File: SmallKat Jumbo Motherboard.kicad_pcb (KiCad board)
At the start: 4 copper layers, 80 x 80 mm, 49 parts, among them IC1 TPS562201DDCR, IC2 TPS562201DDCR, J1 Conn_01x06_Male, J10 Conn_01x06_Male, J11 Conn_01x06_Male, J12 Conn_01x05_Male, J13 Conn_01x02_Male, J14 Conn_01x04_Male, J15 Conn_01x04_Male, J16 Conn_01x06_Male, J2 Conn_01x06_Male, J3 Conn_01x06_Male, J4 Conn_01x06_Male, J5 Conn_01x06_Male, J6 Conn_01x06_Male, J7 Conn_01x06_Male, J8 Conn_01x06_Male, J9 Conn_01x06_Male, U1 STM32H753IITx, Y1 32.768khz, Y2 32MHZ

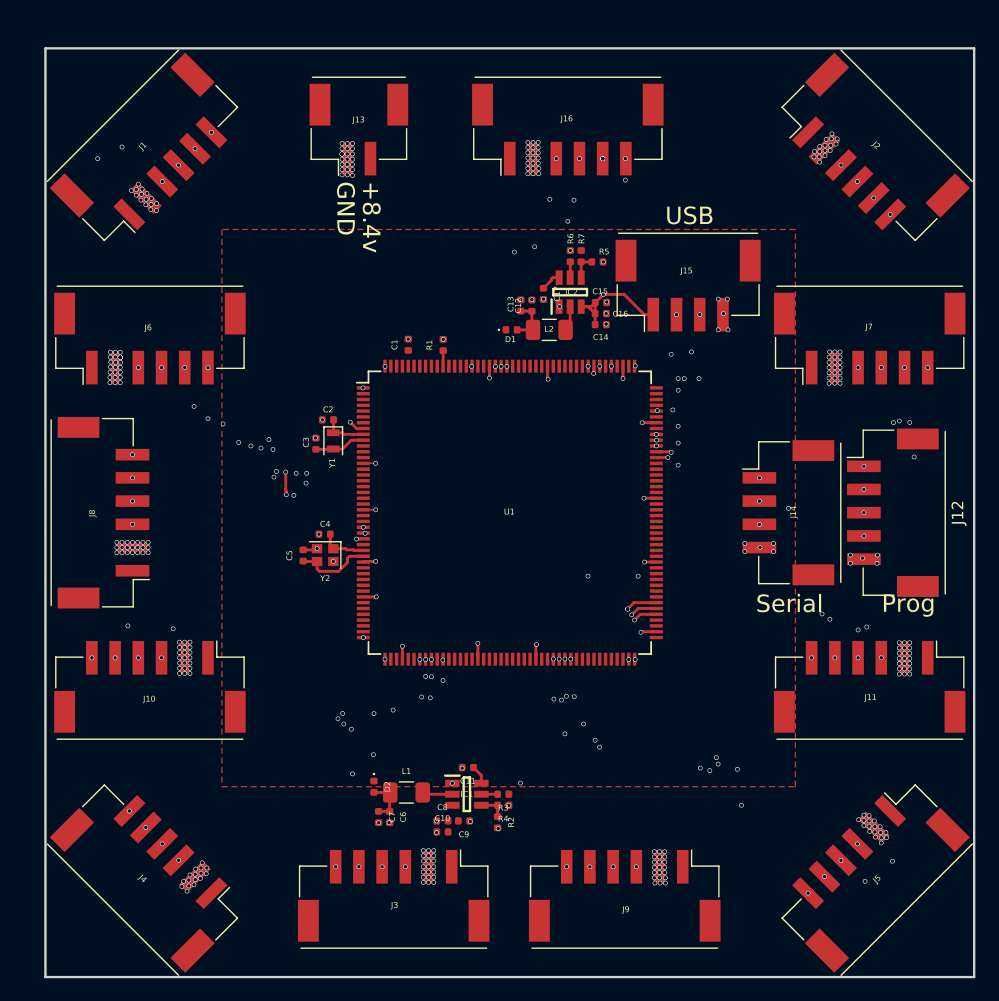
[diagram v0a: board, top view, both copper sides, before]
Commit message: Rev 2
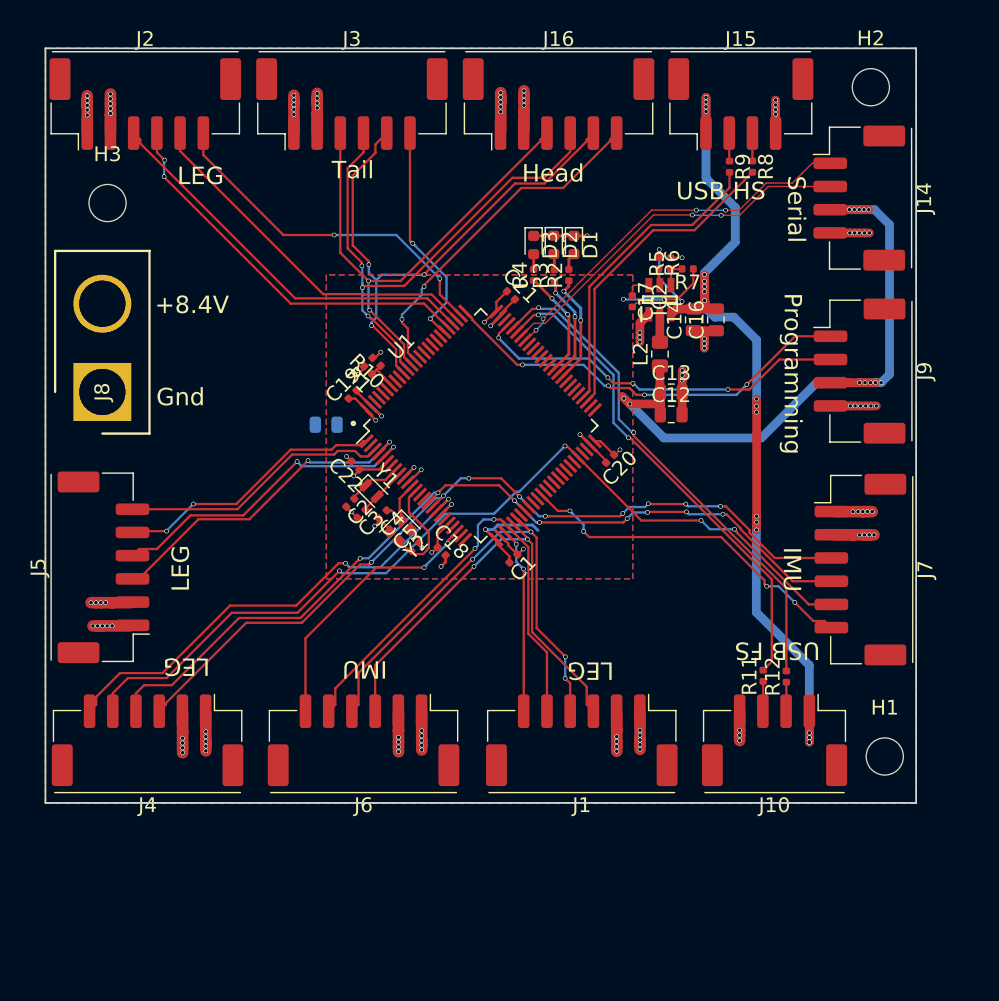
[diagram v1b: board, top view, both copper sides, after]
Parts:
- removed C10, C11: 0.1UF, Capacitor_SMD:C_0402_1005Metric
- removed C15, C8, C9: 10UF, Capacitor_SMD:C_0402_1005Metric
- removed C6, C7: 22UF, Capacitor_SMD:C_0402_1005Metric
- removed IC1: TPS562201DDCR, TPS562201DDCR:SOT95P280X110-6N
- removed J11: Conn_01x06_Male, Connector_Molex:Molex_CLIK-Mate_502443-0670_1x06-1MP_P2.00mm_Vertical
- removed J12: Conn_01x05_Male, Connector_Molex:Molex_CLIK-Mate_502443-0570_1x05-1MP_P2.00mm_Vertical
- removed J13: Conn_01x02_Male, Connector_Molex:Molex_CLIK-Mate_502443-0270_1x02-1MP_P2.00mm_Vertical
- removed L1: 4.7UH, Inductor_SMD:L_1206_3216Metric
- added C18: 0.1uF, Capacitor_SMD:C_0402_1005Metric, F.Cu at (34.1, 43.3)
- added C19: 0.1uF, Capacitor_SMD:C_0402_1005Metric, F.Cu at (26.5, 29.8)
- added C20: 0.1uF, Capacitor_SMD:C_0402_1005Metric, F.Cu at (48.6, 35.4)
- added C21: 0.1uF, Capacitor_SMD:C_0402_1005Metric, F.Cu at (40.1, 21.3)
- added C22: 0.1uF, Capacitor_SMD:C_0402_1005Metric, F.Cu at (26.7, 35.9)
- added D3: LED, LED_SMD:LED_0603_1608Metric, F.Cu at (42.1, 16.9)
- added FB1: Ferrite_Bead, Inductor_SMD:L_0805_2012Metric, B.Cu at (24.2, 32.4)
- added H1: MountingHole, MountingHole:MountingHole_3.2mm_M3, F.Cu at (72.3, 61.0)
- added H2: MountingHole, MountingHole:MountingHole_3.2mm_M3, F.Cu at (71.1, 3.35)
- added H3: MountingHole, MountingHole:MountingHole_3.2mm_M3, F.Cu at (5.35, 13.3)
- added R10: 10k, Resistor_SMD:R_0402_1005Metric, F.Cu at (28.5, 27.0)
- added R11: 33R, Resistor_SMD:R_0402_1005Metric, F.Cu at (61.8, 54.0)
- added R12: 33R, Resistor_SMD:R_0402_1005Metric, F.Cu at (63.8, 54.1)
- added R8: 33R, Resistor_SMD:R_0402_1005Metric, F.Cu at (60.9, 10.2)
- added R9: 33R, Resistor_SMD:R_0402_1005Metric, F.Cu at (58.9, 10.2)
- C1: value 1UF -> 0.1uF
- C12, C13, C14, C16: footprint Capacitor_SMD:C_0402_1005Metric -> Capacitor_SMD:C_0805_2012Metric
- D1, D2: value 641-1675-1-ND -> LED; footprint Diode_SMD:D_0402_1005Metric -> LED_SMD:LED_0603_1608Metric
- J10, J9: value Conn_01x06_Male -> Conn_01x04_Male; footprint Connector_Molex:Molex_CLIK-Mate_502443-0670_1x06-1MP_P2.00mm_Vertical -> Connector_Molex:Molex_CLIK-Mate_502443-0470_1x04-1MP_P2.00mm_Vertical
- J8: value Conn_01x06_Male -> PRT-10474; footprint Connector_Molex:Molex_CLIK-Mate_502443-0670_1x06-1MP_P2.00mm_Vertical -> PRT-10474:SHDR2W320P716_1X2_1574X813X1588P
- L2: footprint Inductor_SMD:L_1206_3216Metric -> Inductor_SMD:L_0805_2012Metric_Pad1.15x1.40mm_HandSolder
- R1, R5: value 10K -> 10k
- R2, R3: value 10K -> 330R
- R4: value 33.2K -> 330R
- R7: value 33.2K -> 33.2k
- U1: value STM32H753IITx -> STM32H743VITx; footprint Package_QFP:LQFP-176_24x24mm_P0.5mm -> Package_QFP:LQFP-100_14x14mm_P0.5mm
- moved J5 71.0 mm to (5.00, 44.7), turned to 90 degrees
- moved J3 68.3 mm to (26.4, 4.80), turned to 0 degrees
- moved J1 62.8 mm to (46.2, 59.6), turned to 180 degrees
- moved J2 62.5 mm to (8.60, 4.80), turned to 0 degrees
- moved J10 54.0 mm to (62.8, 59.6)
- moved J9 49.5 mm to (70.1, 27.8), turned to 270 degrees
- moved D2 49.2 mm to (43.8, 16.9)
- moved R2 47.5 mm to (45.1, 19.5), turned to 90 degrees
- moved R4 45.8 mm to (42.1, 19.5), turned to 90 degrees
- moved R3 44.9 mm to (43.8, 19.6), turned to 90 degrees
- moved J6 39.2 mm to (27.4, 59.6), turned to 180 degrees
- moved J14 27.8 mm to (70.1, 12.9)
- moved C1 20.5 mm to (40.3, 44.0), turned to 225 degrees
- moved J7 19.9 mm to (70.2, 44.9), turned to 270 degrees
- moved J15 16.3 mm to (59.9, 4.80)
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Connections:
- C1 pad 2: GND -> MCU_GND
- C12 pad 1: Net-(C12-Pad1) -> +3V3
- C13 pad 1: Net-(C12-Pad1) -> +3V3
- C17 pad 2: GND -> Net-(C17-Pad2)
- C2 pad 2: GND -> MCU_GND
- C3 pad 2: GND -> MCU_GND
- C4 pad 2: GND -> MCU_GND
- C5 pad 2: GND -> MCU_GND
- D1 pad 1: +3V3 -> GND
- D1 pad 2: Net-(C12-Pad1) -> Net-(D1-Pad2)
- D2 pad 1: +3V3 -> GND
- D2 pad 2: Net-(C6-Pad1) -> Net-(D2-Pad2)
- IC2 pad 2: Net-(IC2-Pad2) -> Net-(C17-Pad2)
- J1 pad 3: SCK1 -> MISO1
- J1 pad 4: MISO1 -> MOSI1
- J1 pad 5: MOSI1 -> SCK1
- J1 pad 6: CS1_1 -> CS1
- J10 pad 1: +BATT -> +5V
- J10 pad 2: GND -> Net-(J10-Pad2)
- J10 pad 3: SCK5 -> Net-(J10-Pad3)
- J10 pad 4: MISO5 -> GND
- J15 pad 2: USBDM -> Net-(J15-Pad2)
- J15 pad 3: USBDP -> Net-(J15-Pad3)
- J16 pad 6: CS6 -> CS6_HEAD
- J2 pad 3: SCK1 -> MISO3
- J2 pad 4: MISO1 -> MOSI3
- J2 pad 5: MOSI1 -> SCK3
- J2 pad 6: CS1_2 -> CS3
- J3 pad 3: SCK2 -> SCK6
- J3 pad 4: MISO2 -> MISO6
- J3 pad 5: MOSI2 -> MOSI6
- J3 pad 6: CS2 -> CS6_TAIL
- J4 pad 3: SCK1 -> MISO2
- J4 pad 4: MISO1 -> MOSI2
- J4 pad 5: MOSI1 -> SCK2
- J4 pad 6: CS1_3 -> CS2
- J5 pad 3: SCK1 -> MISO4
- J5 pad 4: MISO1 -> MOSI4
- J5 pad 5: MOSI1 -> SCK4
- J5 pad 6: CS1_4 -> CS4
- J6 pad 3: SCK5 -> MISO1
- J6 pad 4: MISO5 -> MOSI1
- J6 pad 5: MOSI5 -> SCK1
- J6 pad 6: CS5_1 -> IMU1_CS
- J7 pad 3: SCK5 -> MISO2
- J7 pad 4: MISO5 -> MOSI2
- J7 pad 5: MOSI5 -> SCK2
- J7 pad 6: CS5_2 -> IMU2_CS
- J8 pad 1: +BATT -> GND
- J8 pad 2: GND -> +BATT
- J9 pad 1: +BATT -> SWCLK
- J9 pad 2: GND -> SWDIO
- J9 pad 3: SCK4 -> +3V3
- J9 pad 4: MISO4 -> GND
- L2 pad 1: Net-(C12-Pad1) -> +3V3
- L2 pad 2: Net-(IC2-Pad2) -> Net-(C17-Pad2)
- R2 pad 1: Net-(IC1-Pad4) -> LED1
- R2 pad 2: GND -> Net-(D1-Pad2)
- R3 pad 1: +BATT -> LED2
- R3 pad 2: Net-(IC1-Pad5) -> Net-(D2-Pad2)
- R4 pad 1: +3V3 -> LED3
- R4 pad 2: Net-(IC1-Pad4) -> Net-(D3-Pad2)
- U1 pad 1: CS5_1 -> SCK4
- U1 pad 10: OSCOUT_32 -> MCU_GND
- U1 pad 100: (no net) -> +3V3
- U1 pad 11: (no net) -> +3V3
- U1 pad 12: (no net) -> OSCIN
- U1 pad 13: (no net) -> OSCOUT
- U1 pad 14: GND -> Net-(U1-Pad14)
- U1 pad 15: +3V3 -> Net-(U1-Pad15)
- U1 pad 16: (no net) -> MOSI2
- U1 pad 17: (no net) -> MISO2
- U1 pad 18: (no net) -> CS2
- U1 pad 19: (no net) -> MCU_GND
- U1 pad 2: (no net) -> Net-(U1-Pad2)
- U1 pad 20: (no net) -> Net-(U1-Pad20)
- U1 pad 21: (no net) -> +3V3
- U1 pad 22: GND -> Net-(U1-Pad22)
- U1 pad 23: +3V3 -> IMU1_CS
- U1 pad 24: (no net) -> Net-(U1-Pad24)
- U1 pad 25: SCK5 -> Net-(U1-Pad25)
- U1 pad 26: MISO5 -> MCU_GND
- U1 pad 27: MOSI5 -> +3V3
- U1 pad 28: (no net) -> CS1
- U1 pad 29: OSCIN -> SCK1
- U1 pad 3: (no net) -> CS4
- U1 pad 30: OSCOUT -> MISO1
- U1 pad 31: NRST -> MOSI1
- U1 pad 32: (no net) -> Net-(U1-Pad32)
- U1 pad 33: (no net) -> Net-(U1-Pad33)
- U1 pad 34: (no net) -> Net-(U1-Pad34)
- U1 pad 35: (no net) -> Net-(U1-Pad35)
- U1 pad 36: +3V3 -> Net-(U1-Pad36)
- U1 pad 37: GND -> IMU2_CS
- U1 pad 38: (no net) -> Net-(U1-Pad38)
- U1 pad 39: +3V3 -> Net-(U1-Pad39)
- U1 pad 4: (no net) -> MISO4
- U1 pad 40: (no net) -> Net-(U1-Pad40)
- U1 pad 41: (no net) -> Net-(U1-Pad41)
- U1 pad 42: (no net) -> Net-(U1-Pad42)
- U1 pad 43: (no net) -> Net-(U1-Pad43)
- U1 pad 44: CS5_3 -> Net-(U1-Pad44)
- U1 pad 45: CS1_3 -> Net-(U1-Pad45)
- U1 pad 46: (no net) -> SCK2
- U1 pad 47: (no net) -> Net-(U1-Pad47)
- U1 pad 48: GND -> Net-(U1-Pad48)
- U1 pad 49: +3V3 -> MCU_GND
- U1 pad 5: (no net) -> MOSI4
- U1 pad 50: (no net) -> +3V3
- U1 pad 51: SCK1 -> Net-(U1-Pad51)
- U1 pad 52: MISO1 -> Net-(U1-Pad52)
- U1 pad 53: MOSI1 -> USB_HS_N
- U1 pad 54: (no net) -> USB_HS_P
- U1 pad 55: CS2 -> Net-(U1-Pad55)
- U1 pad 56: (no net) -> Net-(U1-Pad56)
- U1 pad 57: (no net) -> Net-(U1-Pad57)
- U1 pad 58: (no net) -> Net-(U1-Pad58)
- U1 pad 59: (no net) -> LED1
- U1 pad 6: (no net) -> +3V3
- U1 pad 60: (no net) -> LED2
- U1 pad 61: GND -> LED3
- U1 pad 62: +3V3 -> Net-(U1-Pad62)
- U1 pad 63: (no net) -> Net-(U1-Pad63)
- U1 pad 64: (no net) -> Net-(U1-Pad64)
- U1 pad 65: (no net) -> Net-(U1-Pad65)
- U1 pad 66: (no net) -> Net-(U1-Pad66)
- U1 pad 67: (no net) -> Net-(U1-Pad67)
- U1 pad 68: (no net) -> TX
- U1 pad 69: (no net) -> RX
- U1 pad 7: (no net) -> Net-(U1-Pad7)
- U1 pad 70: (no net) -> USB_FS_N
- U1 pad 71: GND -> USB_FS_P
- U1 pad 72: +3V3 -> SWDIO
- U1 pad 73: (no net) -> Net-(U1-Pad73)
- U1 pad 74: CS4 -> MCU_GND
- U1 pad 75: SCK4 -> +3V3
- U1 pad 76: MISO4 -> SWCLK
- U1 pad 77: MOSI4 -> CS3
- U1 pad 78: (no net) -> SCK3
- U1 pad 79: (no net) -> MISO3
- U1 pad 8: CS3 -> OSCIN_32
- U1 pad 80: (no net) -> MOSI3
- U1 pad 81: (no net) -> CS6_TAIL
- U1 pad 82: +3V3 -> Net-(U1-Pad82)
- U1 pad 83: (no net) -> Net-(U1-Pad83)
- U1 pad 84: (no net) -> Net-(U1-Pad84)
- U1 pad 85: (no net) -> Net-(U1-Pad85)
- U1 pad 86: (no net) -> Net-(U1-Pad86)
- U1 pad 87: CS1_4 -> Net-(U1-Pad87)
- U1 pad 88: CS5_4 -> CS6_HEAD
- U1 pad 89: (no net) -> SCK6
- U1 pad 9: OSCIN_32 -> OSCOUT_32
- U1 pad 90: GND -> MISO6
- U1 pad 91: +3V3 -> MOSI6
- U1 pad 92: (no net) -> CS6
- U1 pad 93: SCK2 -> Net-(U1-Pad93)
- U1 pad 94: MISO2 -> Net-(R1-Pad1)
- U1 pad 95: MOSI2 -> Net-(U1-Pad95)
- U1 pad 96: (no net) -> Net-(U1-Pad96)
- U1 pad 97: (no net) -> Net-(U1-Pad97)
- U1 pad 98: (no net) -> Net-(U1-Pad98)
- U1 pad 99: (no net) -> MCU_GND
- Y2 pad 2: GND -> MCU_GND
- Y2 pad 4: GND -> MCU_GND
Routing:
- net SCK1: track 221.0 -> 41.7 mm, vias 11 -> 2
- net MISO1: track 218.4 -> 40.6 mm, vias 11 -> 2
- net MOSI1: track 215.5 -> 41.9 mm, vias 9 -> 4
- net SCK5: track 122.8 -> 0.00 mm, vias 13 -> 0
- net MISO5: track 119.8 -> 0.00 mm, vias 14 -> 0
- net MOSI5: track 116.8 -> 0.00 mm, vias 8 -> 0
- net +3V3: track 11.7 -> 87.1 mm, vias 4 -> 22
- net +5V: track 15.7 -> 85.3 mm, vias 2 -> 21
- net NRST: track 47.9 -> 0.00 mm, vias 5 -> 0
- net USB_FS_P: track 0.00 -> 43.9 mm, vias 0 -> 2
- net USB_FS_N: track 0.00 -> 42.6 mm, vias 0 -> 2
- net GND: track 16.3 -> 56.1 mm, vias 309 -> 65
- net SCK2: track 45.6 -> 78.1 mm, vias 2 -> 4
- net IMU2_CS: track 0.00 -> 30.2 mm, vias 0 -> 4
- net CS6_HEAD: track 0.00 -> 29.9 mm, vias 0 -> 2
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- added copper zone on In1.Cu, net +3V3
- added copper zone on In1.Cu, net +BATT
- added copper zone on In2.Cu, net GND
- added copper zone on B.Cu, net MCU_GND
- removed copper zone on In2.Cu, net +BATT
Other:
- board size 80 x 80 mm -> 75 x 65 mm
- board text added: "+8.4V"
- board text added: "Gnd"
- board text added: "Head"
- board text added: "IMU"
- board text added: "Keion Bisland"
- board text added: "LEG"
- board text added: "Programming"
- board text added: "SmallKat MQP Motherboard"
- board text added: "Tail"
- board text added: "USB FS"
- board text added: "USB HS"
- board text added: "rev2"
- board text removed: "+8.4v"
- board text removed: "GND"
- board text removed: "Keion Bisland Xavier Little Alex Tacescu"
- board text removed: "Prog"
- board text removed: "SmallKat MQP Motherboard Rev. 1"
- board text removed: "USB"
